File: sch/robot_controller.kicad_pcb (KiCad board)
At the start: 2 copper layers, 100 x 90 mm, 119 parts, among them IC1 ADM3058EBRIZ-RL, IC2 ADM3058EBRIZ-RL, IC3 74LVC2G125DP,125, IC4 74LVC2G125DP,125, IC5 ADM3058EBRIZ-RL, J1 USB_C_Receptacle_USB2.0, J10 Conn_01x03, J11 Conn_01x03, J12 Conn_01x03, J13 Conn_01x04, J14 Conn_01x04, J15 Conn_01x04, J16 Conn_01x02, J17 Conn_01x04, J18 Conn_01x04, J19 Conn_01x03, J2 Conn_01x06, J20 Conn_01x02, J21 Conn_01x03, J22 Conn_01x02, J23 Conn_02x03_Odd_Even, J3 RJ45_LED, J4 Conn_01x06, J5 Conn_01x03, J6 Conn_01x03, J7 Conn_01x03, J8 Conn_01x03, J9 Conn_01x03, Q1 2SC4116, Q2 2SC4116, Q3 IRLML6402, Q4 IRLML6402, U1 Teensy4.1_simple, U2 AZ1117-3.3, U3 ISO1540, U4 NCP718xSN500, U5 LD1117S50TR_SOT223

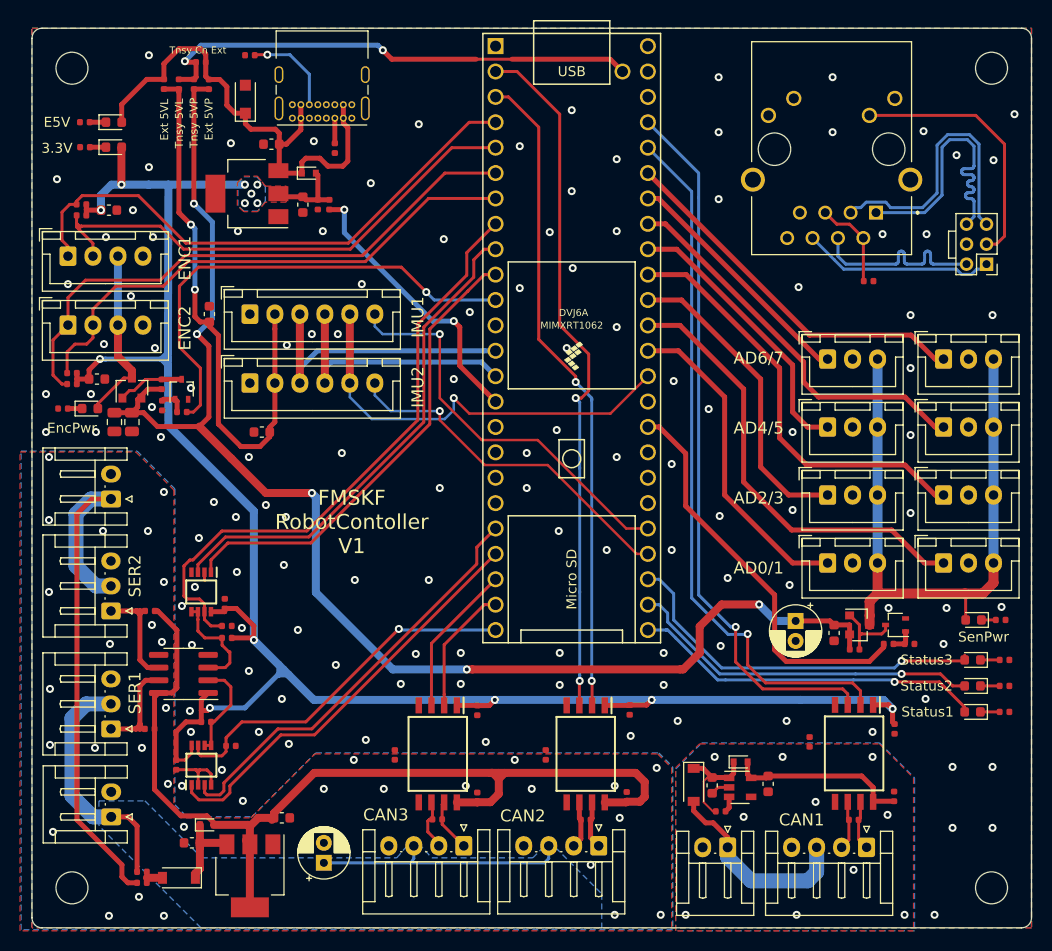
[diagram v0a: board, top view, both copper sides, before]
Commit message: update : sch
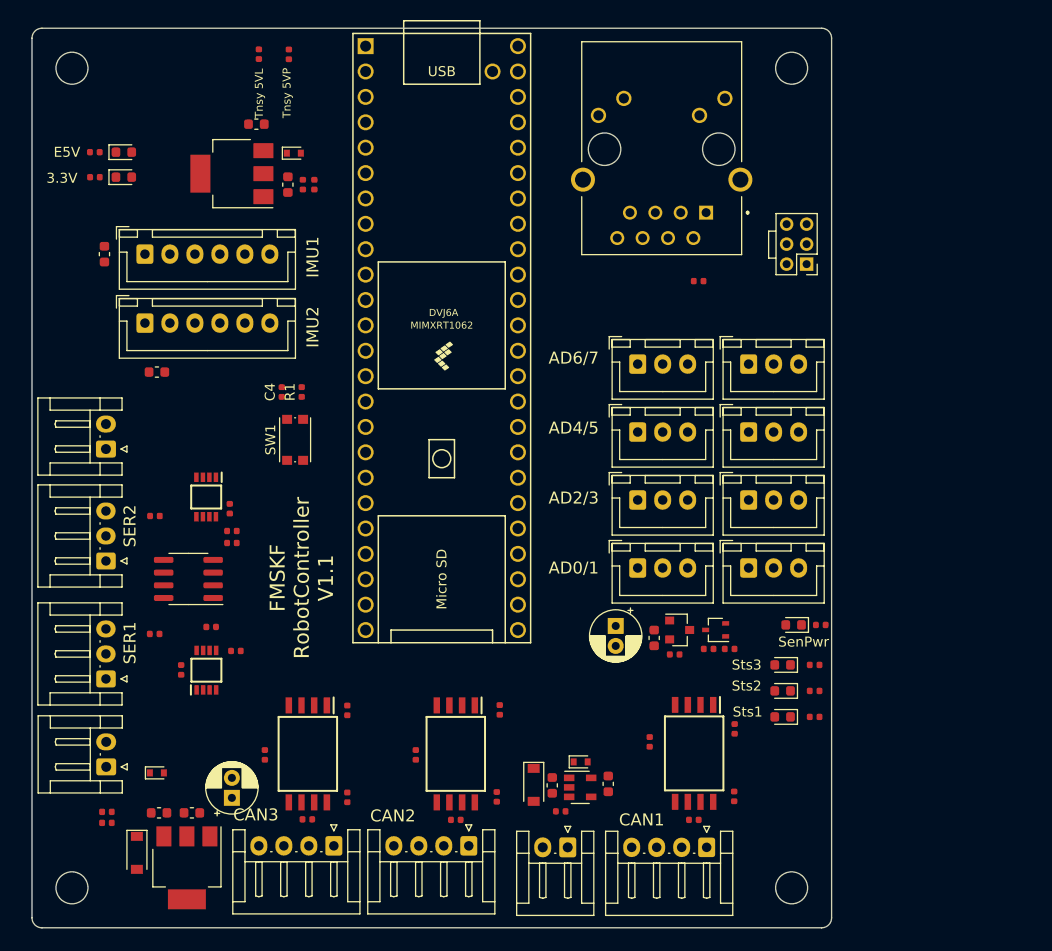
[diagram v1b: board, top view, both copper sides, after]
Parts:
- removed C10, C9: 1u, Capacitor_SMD:C_0603_1608Metric
- removed C23: 22u, Capacitor_SMD:C_0805_2012Metric
- removed D1: D_Schottky, Diode_SMD:D_SOD-123F
- removed D3: LED, LED_SMD:LED_0603_1608Metric
- removed J1: USB_C_Receptacle_USB2.0, Connector_USB:USB_C_Receptacle_GCT_USB4085
- removed J13, J14: Conn_01x04, Connector_JST:JST_XH_B4B-XH-A_1x04_P2.50mm_Vertical
- removed Q1: 2SC4116, Package_TO_SOT_SMD:SOT-323_SC-70
- removed Q3: IRLML6402, Package_TO_SOT_SMD:SOT-23
- removed R11, R13, R9: 10k, Resistor_SMD:R_0402_1005Metric
- removed R15: 1k, Resistor_SMD:R_0402_1005Metric
- removed R17, R18, R20, R21: 2k, Resistor_SMD:R_0402_1005Metric
- removed R2: 5.1k, Resistor_SMD:R_0402_1005Metric
- removed R5, R6, R7: 0 N.C., Resistor_SMD:R_0402_1005Metric
- added SW1: SW_SPST, Button_Switch_SMD:SW_Push_1P1T_NO_CK_KMR2, F.Cu at (126.3, 141.2)
- C4: value 22u -> 0.1u; footprint Capacitor_SMD:C_0805_2012Metric -> Capacitor_SMD:C_0402_1005Metric
- R1: value 5.1k -> 10k
- moved R1 24.6 mm to (127.0, 136.4), turned to 90 degrees
- moved H3 20.0 mm to (176.0, 104.0)
- moved H4 20.0 mm to (176.0, 186.0)
- moved J10 19.5 mm to (171.7, 140.4)
- moved J12 19.5 mm to (171.7, 133.6)
- moved J6 19.5 mm to (171.7, 154.0)
- moved J8 19.5 mm to (171.7, 147.2)
- moved D13 19.0 mm to (175.1, 168.9)
- moved D14 19.0 mm to (175.1, 166.3)
- moved D15 19.0 mm to (175.1, 163.7)
- moved J11 19.0 mm to (160.6, 133.6)
- moved J5 19.0 mm to (160.6, 154.0)
- moved J7 19.0 mm to (160.6, 147.2)
- moved J9 19.0 mm to (160.6, 140.4)
- moved R38 19.0 mm to (178.3, 168.9)
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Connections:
- C4 pad 1: +5VP -> +3V3
- C4 pad 2: GND -> /USER_SWITCH
- C6 pad 1: VBUS -> +5VP
- D2 pad 2: VBUS -> +5VP
- D5 pad 1: VBUS -> +5VP
- R1 pad 1: Net-(J1-PadA5) -> GND
- R1 pad 2: GND -> /USER_SWITCH
- R4 pad 1: VBUS -> VCC
- U1 pad 11: /ENC_PWR -> Net-(U1-Pad11)
- U1 pad 16: Net-(U1-Pad16) -> /USER_SWITCH
- U1 pad 4: /ENC1_A -> Net-(U1-Pad4)
- U1 pad 48: Net-(U1-Pad48) -> VCC
- U1 pad 49: VCC -> Net-(U1-Pad49)
- U1 pad 5: /ENC1_B -> Net-(U1-Pad5)
- U1 pad 6: /ENC2_A -> Net-(U1-Pad6)
- U1 pad 7: /ENC2_B -> Net-(U1-Pad7)
- U2 pad 3: VBUS -> +5VP
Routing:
- net +3.3VP: track 205.5 -> 0.00 mm, vias 13 -> 0
- net +5VP: track 139.3 -> 0.00 mm, vias 5 -> 0
- net /5V_P3: track 97.4 -> 0.00 mm
- net /CAN1_RX: track 71.6 -> 0.00 mm, vias 1 -> 0
- net /CAN1_TX: track 70.9 -> 0.00 mm, vias 1 -> 0
- net /CAN2_RX: track 69.6 -> 0.00 mm, vias 2 -> 0
- net /CAN2_TX: track 65.7 -> 0.00 mm, vias 2 -> 0
- net /WALL_VCC: track 64.0 -> 0.00 mm
- net /SERIAL2_EN: track 61.3 -> 0.00 mm
- net /ENC2_A: track 58.1 -> 0.00 mm
- net /VCC_P3-2: track 57.6 -> 0.00 mm
- net +5VL: track 56.1 -> 0.00 mm, vias 2 -> 0
- net /ENC1_A: track 55.9 -> 0.00 mm
- net /ENC2_B: track 53.0 -> 0.00 mm
- net /ENC1_B: track 52.7 -> 0.00 mm
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- removed copper zone on B.Cu, net +3.3VP
- removed copper zone on F.Cu, net +3.3VP
- removed copper zone on B.Cu, net /GND_P1
- removed copper zone on F.Cu, net /GND_P1
- removed copper zone on B.Cu, net /GND_P3
- removed copper zone on F.Cu, net /GND_P3
- removed copper zone on B.Cu, net /VCC_P3
- removed copper zone on B.Cu, net GND
- removed copper zone on F.Cu, net GND
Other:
- board size 100 x 90 mm -> 80 x 90 mm
- board text added: "FMSKF RobotController V1.1"
- board text added: "Sts1"
- board text added: "Sts2"
- board text added: "Sts3"
- board text removed: "ENC1"
- board text removed: "ENC2"
- board text removed: "EncPwr"
- board text removed: "Ext 5VL"
- board text removed: "Ext 5VP"
- board text removed: "FMSKF RobotContoller V1"
- board text removed: "Status1"
- board text removed: "Status2"
- board text removed: "Status3"
- board text removed: "Tnsy Cn Ext"
